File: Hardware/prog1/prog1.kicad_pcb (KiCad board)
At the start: 2 copper layers, 30.5 x 21 mm, 3 parts, among them J1 Conn_01x02_Male

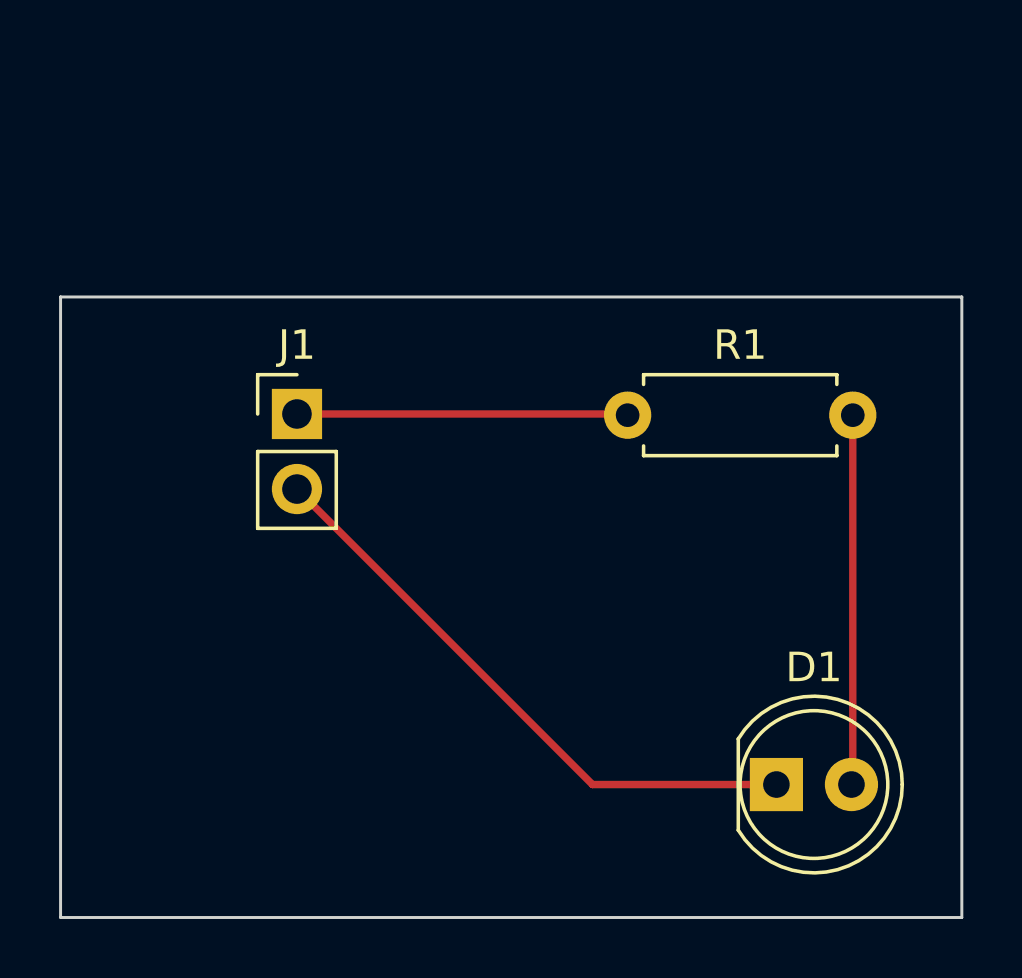
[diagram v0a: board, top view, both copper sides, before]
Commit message: Fix hardware project and firmware project 2
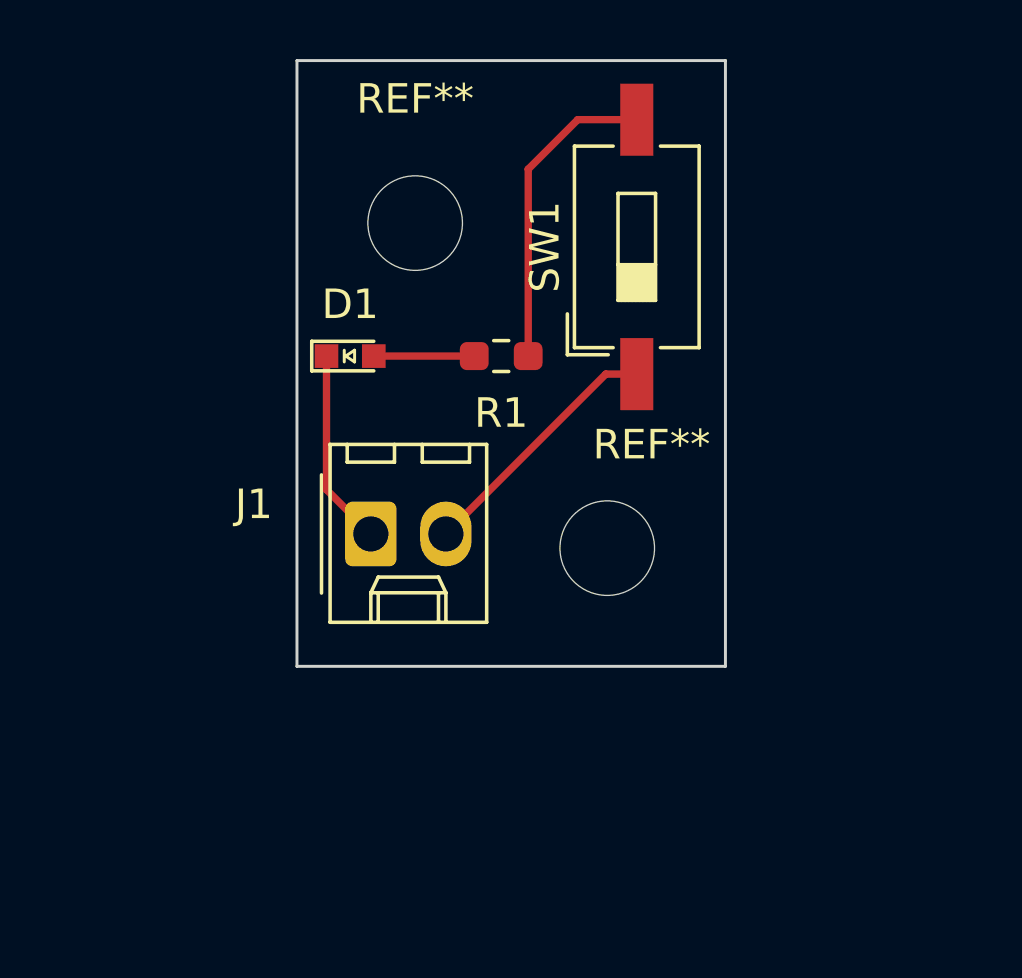
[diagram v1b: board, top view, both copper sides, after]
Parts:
- added REF**: MountingHole_3.2mm_M3, MountingHole:MountingHole_3.2mm_M3, F.Cu at (112.0, 75.0)
- added REF**: MountingHole_3.2mm_M3, MountingHole:MountingHole_3.2mm_M3, F.Cu at (118.5, 86.0)
- added SW1: SW_Push, Button_Switch_SMD:SW_DIP_SPSTx01_Slide_6.7x4.1mm_W8.61mm_P2.54mm_LowProfile, F.Cu at (119.5, 75.8)
- D1: value LED -> LED_RED; footprint LED_THT:LED_D5.0mm -> layout:LED_0603_Symbol_on_F.SilkS
- J1: footprint Connector_PinHeader_2.54mm:PinHeader_1x02_P2.54mm_Vertical -> Connector_Molex:Molex_KK-254_AE-6410-02A_1x02_P2.54mm_Vertical
- R1: value R -> 105; footprint Resistor_THT:R_Axial_DIN0207_L6.3mm_D2.5mm_P7.62mm_Horizontal -> Resistor_SMD:R_0603_1608Metric_Pad0.98x0.95mm_HandSolder
- moved D1 20.5 mm to (109.8, 79.5)
- moved J1 4.77 mm to (110.5, 85.5)
- moved R1 4.72 mm to (114.9, 79.5), turned to 180 degrees
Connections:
- J1 pad 1: +3V3 -> GND
- J1 pad 2: GND -> +3V3
- R1 pad 1: +3V3 -> Net-(R1-Pad1)
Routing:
- net GND: track 20.4 -> 6.64 mm
- net Net-(R1-Pad1): track 0.00 -> 10.7 mm
- net Net-(D1-A): track 12.5 -> 3.40 mm
- net +3V3: track 11.2 -> 8.70 mm
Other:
- board size 30.5 x 21 mm -> 14.5 x 20.5 mm

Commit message: updated hardware project1
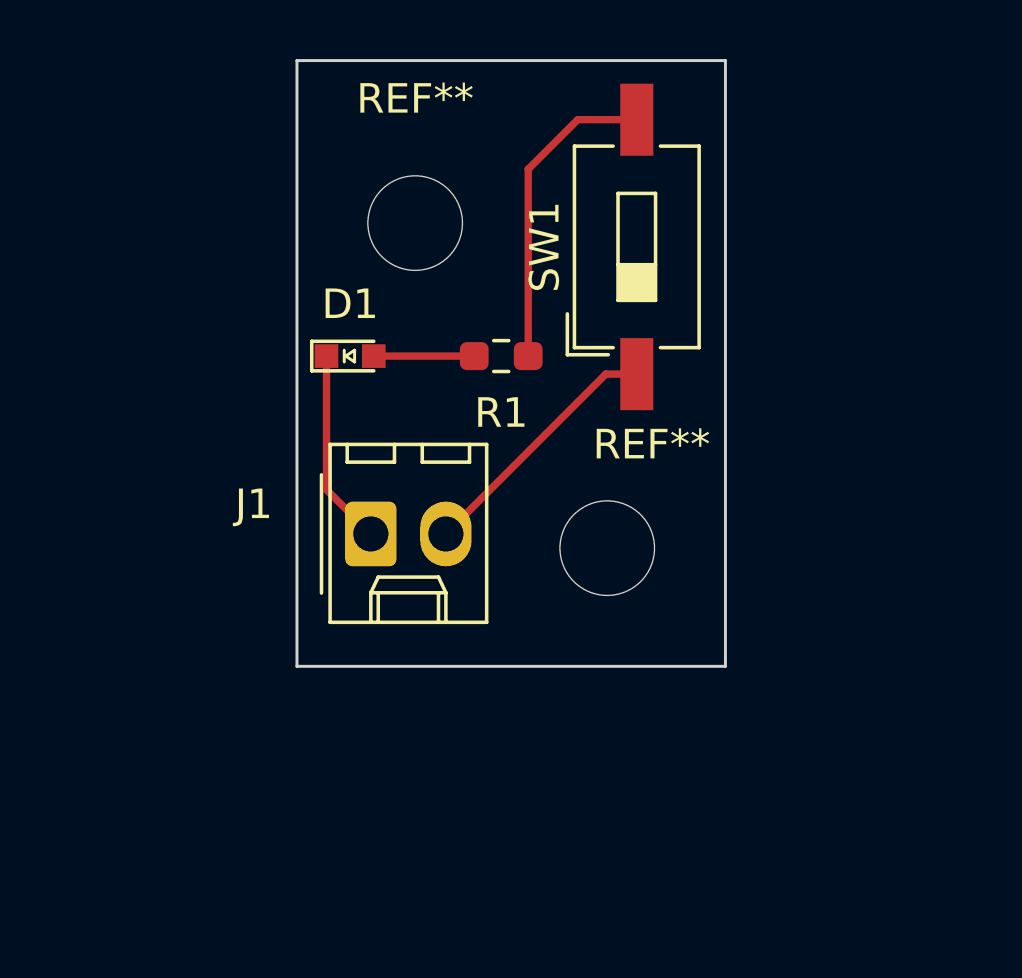
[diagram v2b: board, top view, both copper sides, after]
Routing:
- added copper zone on F.Cu, net GND
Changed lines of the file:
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@@
 		)
 		(fp_text user "${REFERENCE}"
-			(at 2.58 0 360)
+			(at 2.58 0 0)
 			(layer "F.Fab")
 			(effects
@@
 		(net 4)
 	)
+	(zone
+		(net 1)
+		(net_name "GND")
+		(layer "F.Cu")
+		(hatch edge 0.5)
+		(connect_pads
+			(clearance 0.508)
+		)
+		(min_thickness 0.25)
+		(filled_areas_thickness no)
+		(fill yes
+			(thermal_gap 0.5)
+			(thermal_bridge_width 0.5)
+		)
+		(polygon
+			(pts
+				(xy 108 69.5) (xy 122.5 69.5) (xy 122.5 90) (xy 108 90)
+			)
+		)
+	)
 )
